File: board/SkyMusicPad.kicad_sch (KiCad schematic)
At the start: 51 parts, among them SW1 Cherry, SW10 Cherry, SW11 Cherry, SW12 Cherry, SW13 Cherry, SW14 Cherry, SW15 Cherry, SW16 RotaryEncoder_Switch, SW2 Cherry, SW3 Cherry, SW4 Cherry, SW5 Cherry, SW6 Cherry, SW7 Cherry, SW8 Cherry, SW9 Cherry, U1 ESP32-S3-Zero

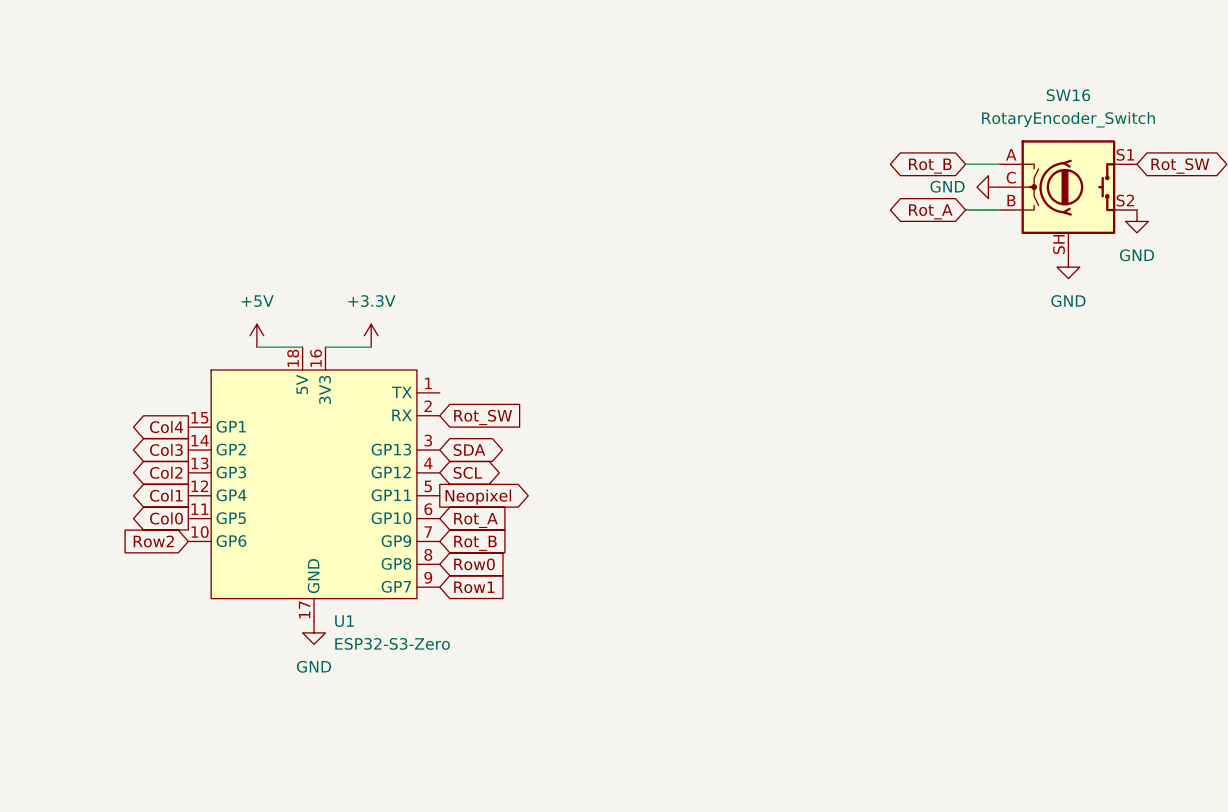
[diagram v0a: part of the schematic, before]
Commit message: Components placed
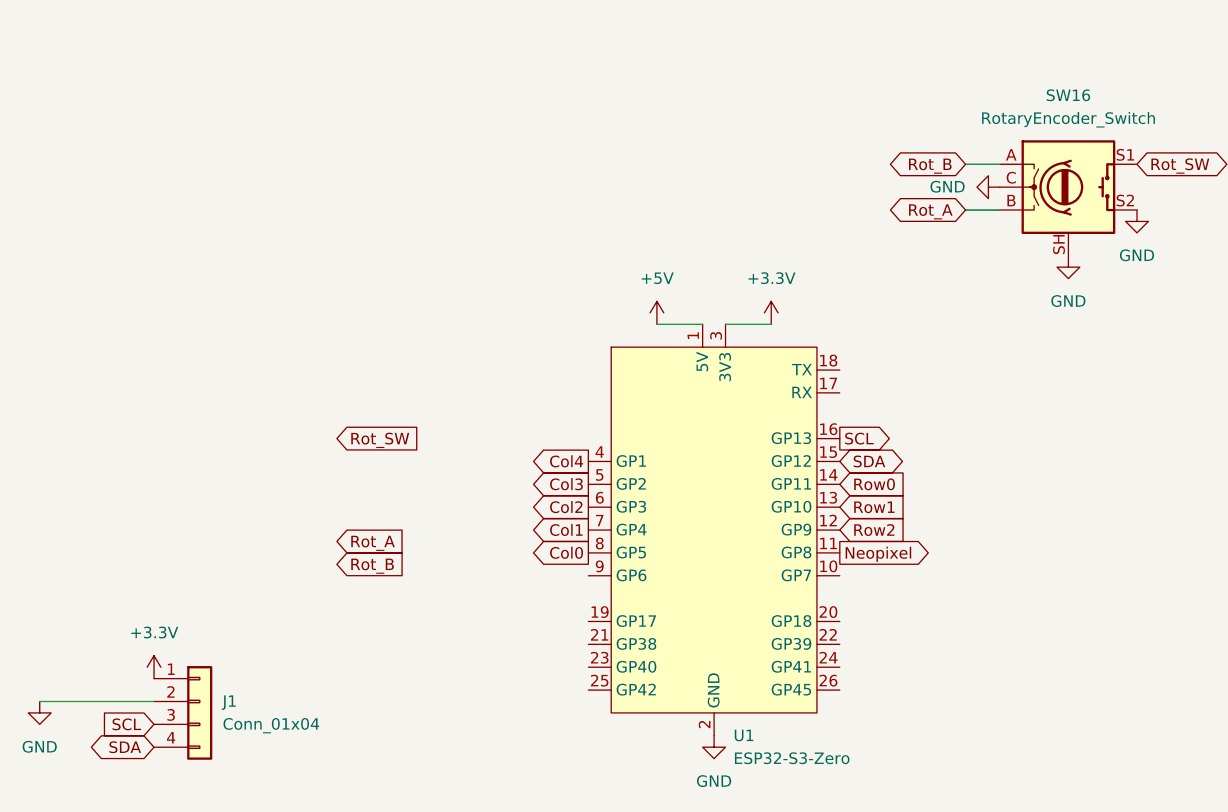
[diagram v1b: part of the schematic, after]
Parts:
- added J1: Conn_01x04, SkyMusic:OLED_DFR0648, symbol Connector_Generic:Conn_01x04
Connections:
- net +3.3V: now also U1.3 (3V3), J1.1 (Pin_1); no longer U1.16 (3V3)
- net +5V: now also U1.1 (5V); no longer U1.18 (5V)
- net Col0: now also U1.8 (GP5); no longer U1.11 (GP5)
- net Col1: now also U1.7 (GP4); no longer U1.12 (GP4)
- net Col2: now also U1.6 (GP3); no longer U1.13 (GP3)
- net Col3: now also U1.5 (GP2); no longer U1.14 (GP2)
- net Col4: now also U1.4 (GP1); no longer U1.15 (GP1)
- net GND: now also U1.2 (GND), J1.2 (Pin_2); no longer U1.17 (GND)
- net Neopixel: now also U1.11 (GP8); no longer U1.5 (GP11)
- net Rot_A: no longer U1.6 (GP10)
- net Rot_B: no longer U1.7 (GP9)
- net Rot_SW: no longer U1.2 (RX)
- net Row0: now also U1.14 (GP11); no longer U1.8 (GP8)
- net Row1: now also U1.13 (GP10); no longer U1.9 (GP7)
- net Row2: now also U1.12 (GP9); no longer U1.10 (GP6)
- net SCL: now also U1.16 (GP13), J1.3 (Pin_3); no longer U1.4 (GP12)
- net SDA: now also U1.15 (GP12), J1.4 (Pin_4); no longer U1.3 (GP13)
